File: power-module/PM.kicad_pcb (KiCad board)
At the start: 4 copper layers, 65 x 34.3 mm, 54 parts, among them J1 Conn_01x01, J2 Conn_01x04, J3 Conn_01x01, J4 Conn_01x16, U2 TAS5825MRHB

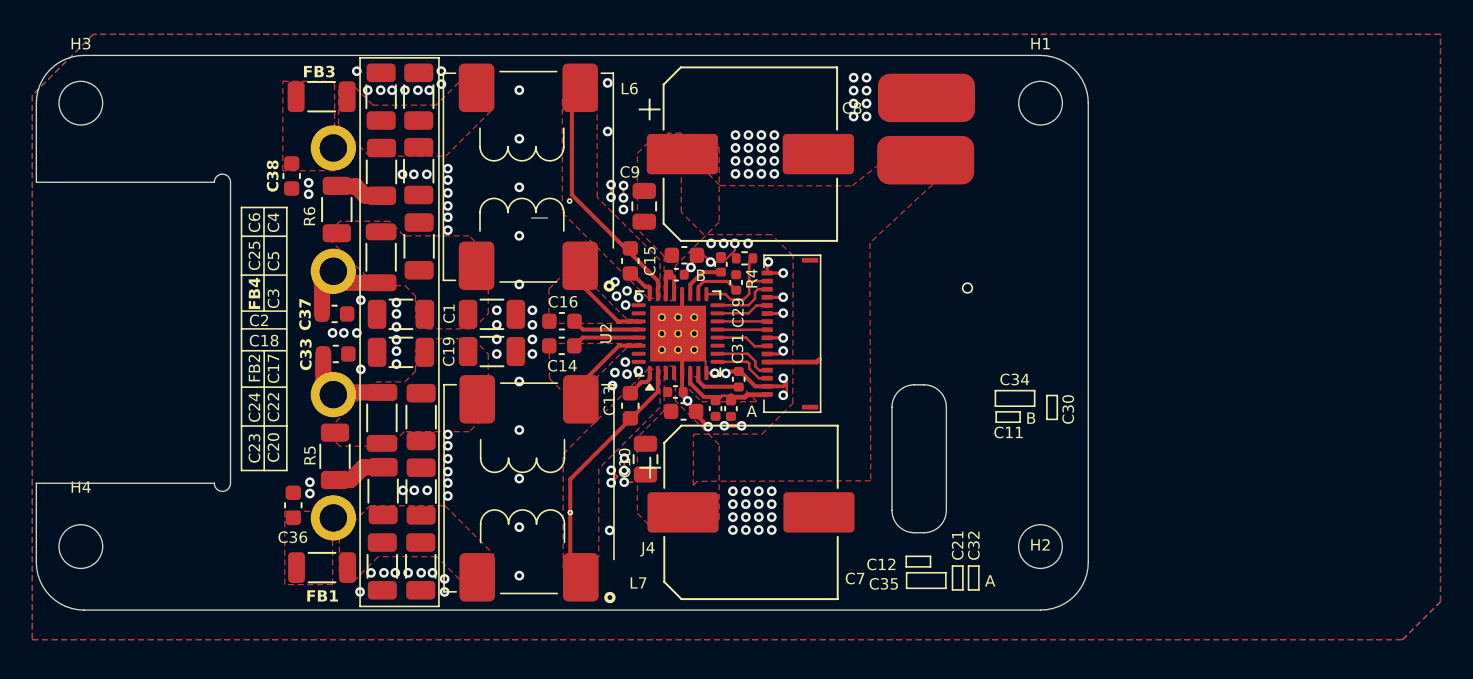
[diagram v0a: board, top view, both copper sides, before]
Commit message: WIP
TODO: Silk PM module. toslink module
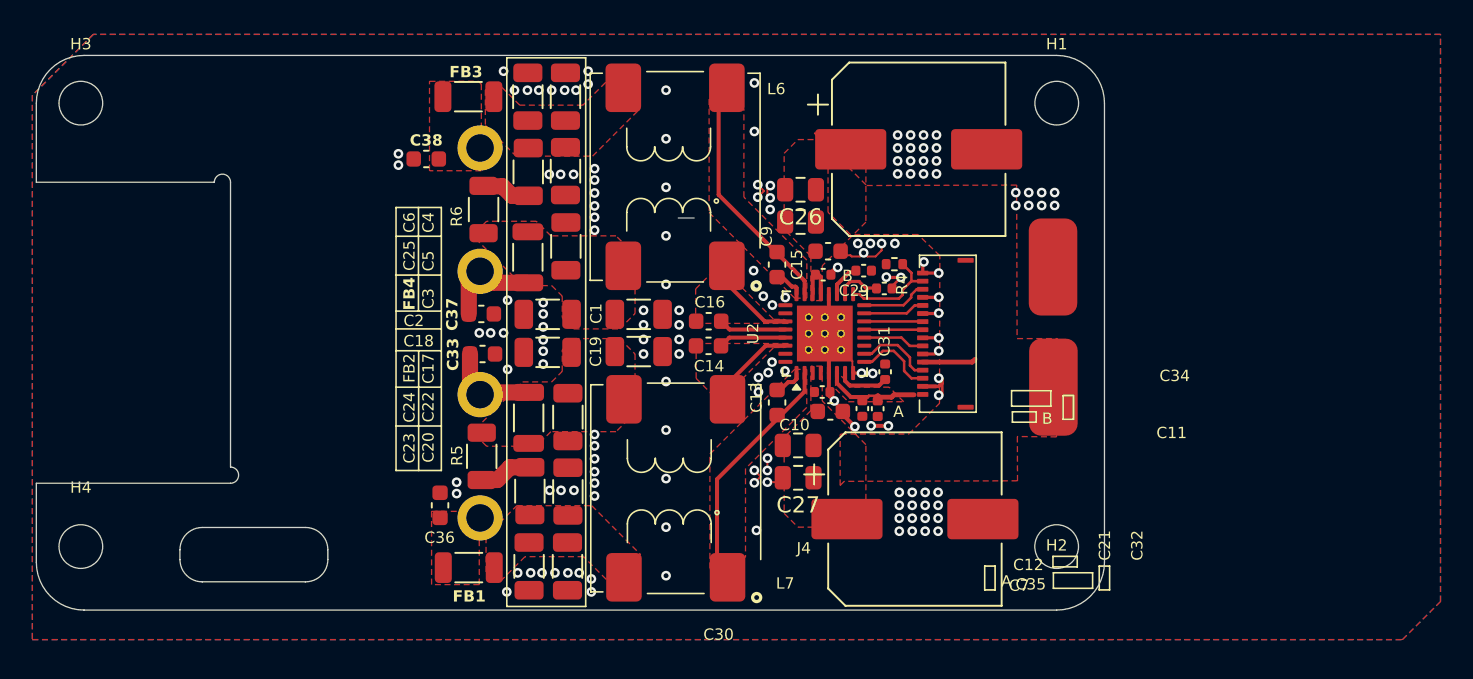
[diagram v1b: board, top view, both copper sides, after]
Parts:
- added C26: 22u, Capacitor_SMD:C_0805_2012Metric, F.Cu at (157.5, 76.6)
- added C27: 22u, Capacitor_SMD:C_0805_2012Metric, F.Cu at (157.4, 94.4)
- moved J1 16.1 mm to (173.1, 88.8), turned to 0 degrees
- moved J3 13.1 mm to (173.1, 81.4), turned to 180 degrees
- moved C8 10.4 mm to (164.8, 74.1)
- moved C7 10.1 mm to (164.6, 97.0)
- moved C9 9.71 mm to (157.5, 78.6), turned to 180 degrees
- moved J4 9.61 mm to (165.1, 85.5)
- moved C10 9.47 mm to (157.4, 92.4), turned to 180 degrees
- moved R4 9.27 mm to (163.3, 81.2)
- moved C29 9.16 mm to (162.7, 82.7), turned to 0 degrees
- moved C13 9.07 mm to (156.1, 89.8)
- moved C15 9.07 mm to (156.1, 81.2)
- moved C1 9.07 mm to (147.5, 84.3)
- moved C11 9.07 mm to (158.9, 81.8)
- moved C12 9.07 mm to (158.8, 89.1)
- moved C14 9.07 mm to (151.8, 86.2)
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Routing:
- net /AMP_IO1: track 3.67 -> 4.94 mm
- net /AMP_IO2: track 3.69 -> 4.77 mm
- net Net-(U2-AVDD): track 2.81 -> 2.12 mm
- net /SDIN: track 3.08 -> 3.62 mm
- net /SCLK: track 3.08 -> 3.62 mm
- net /SDA: track 3.27 -> 3.81 mm
- net /LRCLK: track 3.30 -> 3.82 mm
- net GND: track 38.6 -> 38.5 mm, vias 152 -> 154
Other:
- board size 65 x 34.3 mm -> 66 x 34.3 mm
